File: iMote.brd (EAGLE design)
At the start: 71.6 x 60 mm, 47 parts, among them CN1 C-02235, CN2 ICSP, CN3 CC-HEADER, IC1 ATmega328P-AU, IC2 FT232RLSSOP, IC3 BLE112-A-VISUAL, Q1 16MHz, T1 2SC1815

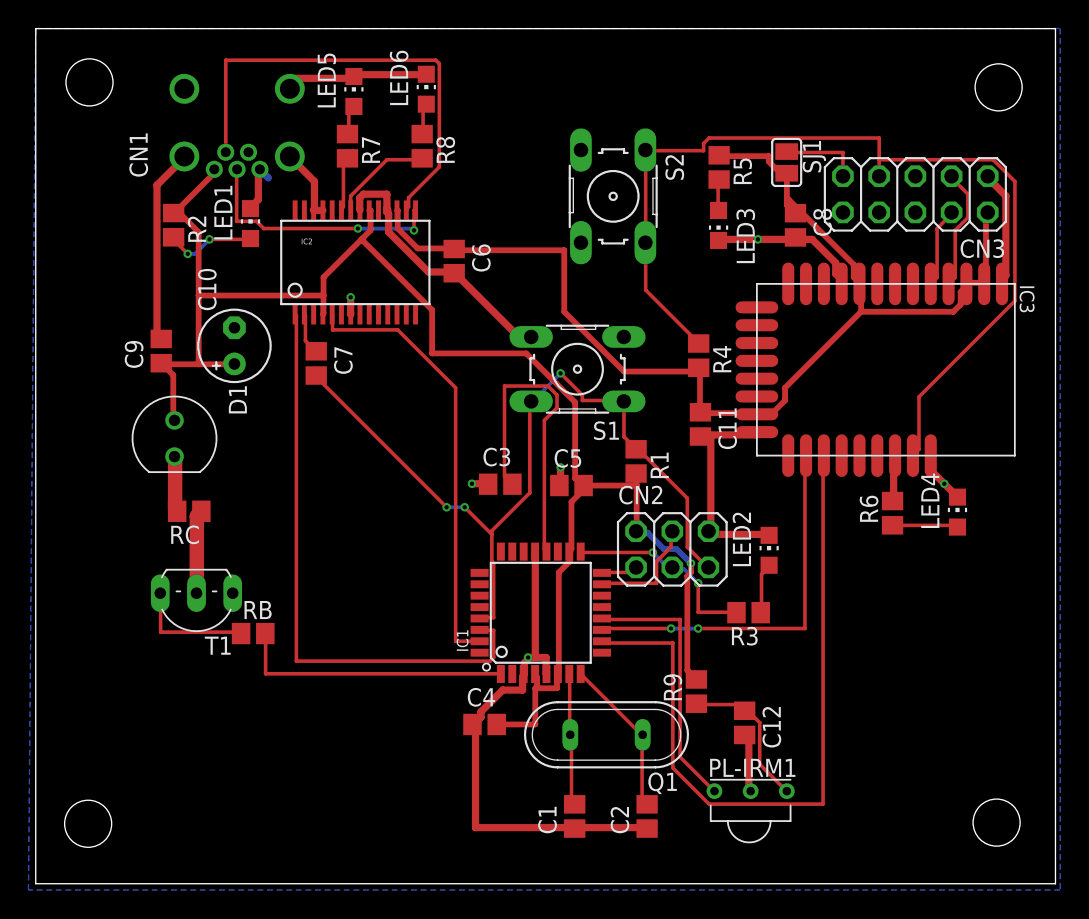
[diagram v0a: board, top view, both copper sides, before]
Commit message: 全部品my.lbr化中
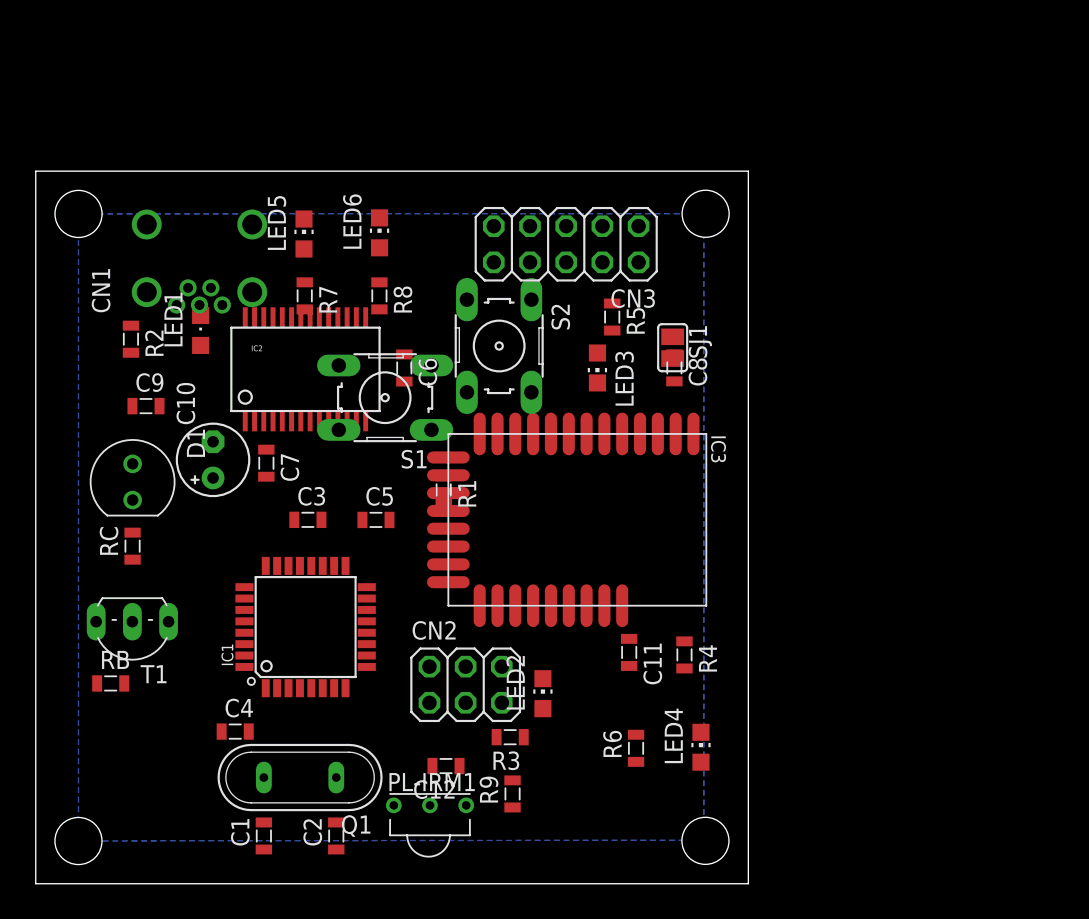
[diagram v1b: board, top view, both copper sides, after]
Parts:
- C1, C11, C12, C2, C3, C4, C5, C6, C7, C8, C9: device rcl:C2012 -> my:2012
- CN1: device akizukidenshi:C-02235 -> my:C-02235
- D1: device akizukidenshi:LED -> my:LED
- IC1: device Arduino-AVR:TQFP32-08 -> my:TQFP32-08
- IC2: device akizukidenshi:SSOP28DB -> my:SSOP28DB
- IC3: device akizukidenshi:BLE112-A -> my:BLE112-A
- LED1: device led:CHIP-LED0805 -> led:CHIPLED_0805
- PL-IRM1: device akizukidenshi:IR-RECEIVER -> my:IR-RECEIVER
- R1, R2, R3, R4, R5, R6, R7, R8, R9, RB, RC: device resistor:R2012 -> my:2012
- moved CN3 24.7 mm to (37.2, 44.9)
- moved LED4 24.4 mm to (46.7, 9.58)
- moved R6 24.4 mm to (42.1, 9.50)
- moved IC3 24.1 mm to (38.0, 25.5)
- moved PL-IRM1 22.5 mm to (27.7, 5.50)
- moved STANDOFF3 22.4 mm to (47.0, 47.0)
- moved C2 21.9 mm to (21.1, 3.35)
- moved C1 21.9 mm to (16.0, 3.35)
- moved Q1 21.7 mm to (18.5, 7.45)
- moved C12 21.2 mm to (28.8, 8.26), turned to 180 degrees
- moved R4 21.0 mm to (45.5, 16.1)
- moved STANDOFF1 20.5 mm to (47.0, 3.01)
- moved R3 18.9 mm to (33.3, 10.3)
- moved LED2 18.8 mm to (35.6, 13.3)
- moved C4 17.5 mm to (14.0, 10.7)
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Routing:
- net GND: track 135.2 -> 0.00 mm, vias 6 -> 0
- net +5V: track 114.6 -> 0.00 mm, vias 1 -> 0
- net +3V3: track 81.7 -> 0.00 mm
- net !BLE/RST: track 67.2 -> 0.00 mm
- net !RESET: track 57.1 -> 0.00 mm, vias 3 -> 0
- net D6/BLERX: track 49.9 -> 0.00 mm
- net D0/USBRX: track 41.2 -> 0.00 mm
- net USBD-: track 32.8 -> 0.00 mm
- net D1/USBTX: track 30.9 -> 0.00 mm
- net D7/BLETX: track 26.5 -> 0.00 mm, vias 2 -> 0
- net AREF: track 22.5 -> 0.00 mm
- net D3/IROUT: track 19.3 -> 0.00 mm
- net D8/IRIN: track 18.6 -> 0.00 mm
- net USBD+: track 17.9 -> 0.00 mm, vias 2 -> 0
- net D13/SCK: track 13.9 -> 0.00 mm, vias 2 -> 0
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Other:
- board size 71.6 x 60 mm -> 50 x 50 mm
